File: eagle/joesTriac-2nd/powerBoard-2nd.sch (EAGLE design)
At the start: 43 parts, among them IC1 7809, IC2 7805, IC3 7909, IC5 7809, IC7 LM311N, J1 XF2E-0815-1, J2 XF2E-0815-1

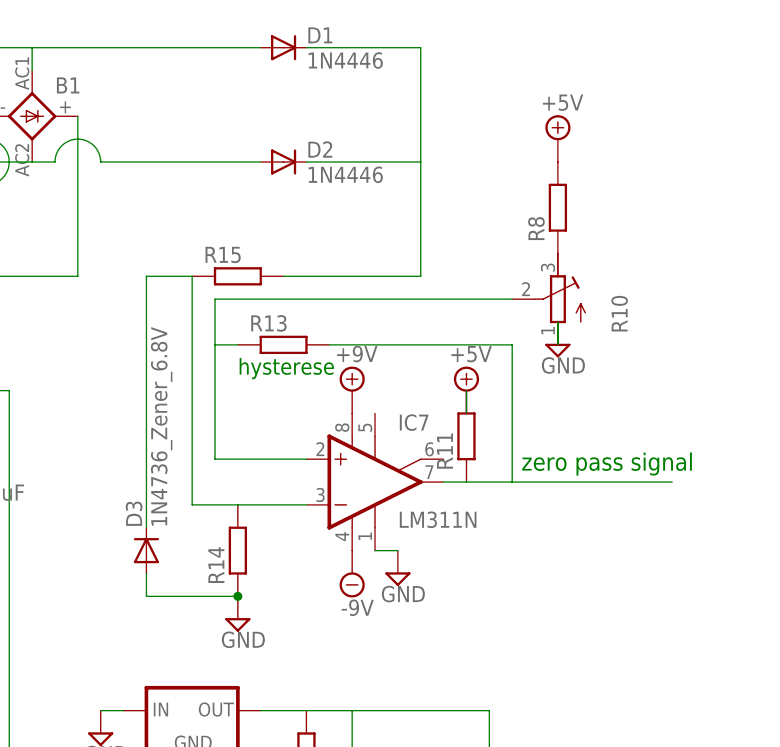
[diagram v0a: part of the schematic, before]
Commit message: reg save
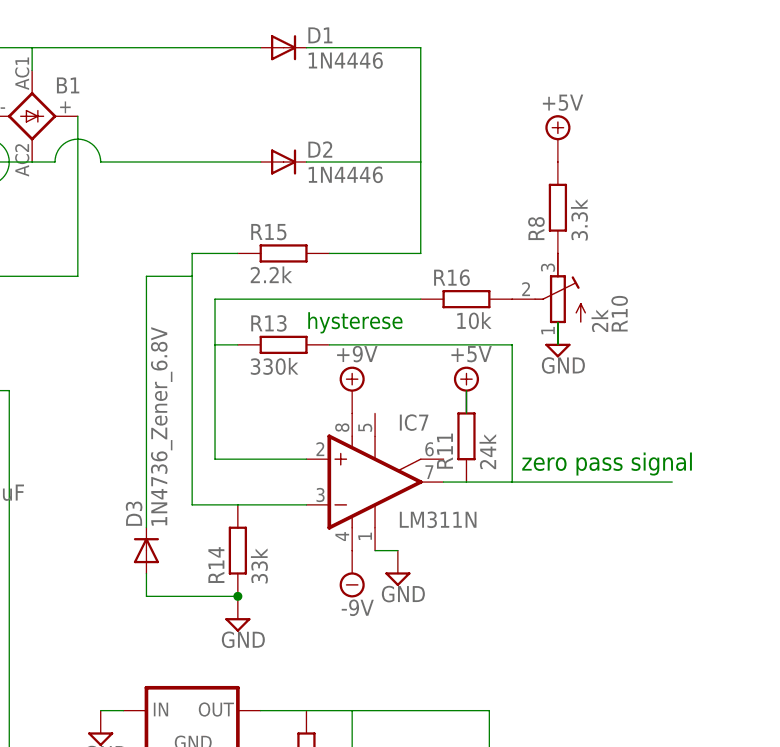
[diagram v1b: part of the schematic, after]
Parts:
- added R16: 10k, resistor:R-EU_0309/V
- R10: value (none) -> 2k
- R11: value (none) -> 24k
- R13: value (none) -> 330k
- R14: value (none) -> 33k
- R15: value (none) -> 2.2k
- R8: value (none) -> 3.3k
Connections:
- new net N$27: R10.S, R16.2
- net N$25: now also R16.1; no longer R10.S
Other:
- moved on the sheet: R15
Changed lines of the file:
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@@
 <part name="D2" library="diode" deviceset="1N4446" device=""/>
 <part name="IC7" library="linear" deviceset="LM311" device="N"/>
-<part name="R8" library="resistor" deviceset="R-EU_" device="0309/V"/>
-<part name="R10" library="resistor" deviceset="R-TRIMM" device="4G/J"/>
+<part name="R8" library="resistor" deviceset="R-EU_" device="0309/V" value="3.3k"/>
+<part name="R10" library="resistor" deviceset="R-TRIMM" device="4G/J" value="2k"/>
 <part name="SUPPLY5" library="supply2" deviceset="+5V" device=""/>
 <part name="SUPPLY17" library="supply2" deviceset="GND" device=""/>
@@
 <part name="SUPPLY19" library="supply2" deviceset="-9V" device=""/>
 <part name="SUPPLY20" library="supply2" deviceset="+5V" device=""/>
-<part name="R11" library="resistor" deviceset="R-EU_" device="0309/V"/>
+<part name="R11" library="resistor" deviceset="R-EU_" device="0309/V" value="24k"/>
 <part name="SUPPLY21" library="supply2" deviceset="GND" device=""/>
-<part name="R13" library="resistor" deviceset="R-EU_" device="0309/V"/>
-<part name="R14" library="resistor" deviceset="R-EU_" device="0309/V"/>
+<part name="R13" library="resistor" deviceset="R-EU_" device="0309/V" value="330k"/>
+<part name="R14" library="resistor" deviceset="R-EU_" device="0309/V" value="33k"/>
 <part name="SUPPLY23" library="supply2" deviceset="GND" device=""/>
-<part name="R15" library="resistor" deviceset="R-EU_" device="0309/V"/>
+<part name="R15" library="resistor" deviceset="R-EU_" device="0309/V" value="2.2k"/>
 <part name="D3" library="diode" deviceset="1N4446" device="" value="1N4736_Zener_6.8V"/>
+<part name="R16" library="resistor" deviceset="R-EU_" device="0309/V" value="10k"/>
 </parts>
 <sheets>
@@
 <text x="-124.46" y="-10.16" size="1.778" layer="91">/-16V</text>
 <text x="46.736" y="46.99" size="1.9304" layer="91">zero pass signal</text>
-<text x="15.24" y="57.658" size="1.778" layer="91">hysterese</text>
+<text x="22.86" y="62.738" size="1.778" layer="91">hysterese</text>
 </plain>
 <instances>
@@
 <instance part="R14" gate="G$1" x="15.24" y="38.1" rot="R90"/>
 <instance part="SUPPLY23" gate="GND" x="15.24" y="30.48"/>
-<instance part="R15" gate="G$1" x="15.24" y="68.58"/>
+<instance part="R15" gate="G$1" x="20.32" y="71.12"/>
 <instance part="D3" gate="1" x="5.08" y="38.1" rot="R90"/>
+<instance part="R16" gate="G$1" x="40.64" y="66.04" smashed="yes">
+<attribute name="NAME" x="36.83" y="67.5386" size="1.778" layer="95"/>
+<attribute name="VALUE" x="39.37" y="62.738" size="1.778" layer="96"/>
+</instance>
 </instances>
 <busses>
@@
 <net name="N$22" class="0">
 <segment>
-<wire x1="10.16" y1="68.58" x2="10.16" y2="43.18" width="0.1524" layer="91"/>
-<wire x1="10.16" y1="43.18" x2="15.24" y2="43.18" width="0.1524" layer="91"/>
+<wire x1="10.16" y1="68.58" x2="5.08" y2="68.58" width="0.1524" layer="91"/>
+<wire x1="5.08" y1="68.58" x2="5.08" y2="40.64" width="0.1524" layer="91"/>
+<pinref part="D3" gate="1" pin="C"/>
 <pinref part="IC7" gate="A" pin="-IN"/>
 <wire x1="15.24" y1="43.18" x2="22.86" y2="43.18" width="0.1524" layer="91"/>
 <pinref part="R14" gate="G$1" pin="2"/>
+<wire x1="10.16" y1="43.18" x2="15.24" y2="43.18" width="0.1524" layer="91"/>
+<wire x1="10.16" y1="68.58" x2="10.16" y2="43.18" width="0.1524" layer="91"/>
 <pinref part="R15" gate="G$1" pin="1"/>
-<wire x1="10.16" y1="68.58" x2="5.08" y2="68.58" width="0.1524" layer="91"/>
-<wire x1="5.08" y1="68.58" x2="5.08" y2="40.64" width="0.1524" layer="91"/>
-<pinref part="D3" gate="1" pin="C"/>
+<wire x1="15.24" y1="71.12" x2="10.16" y2="71.12" width="0.1524" layer="91"/>
+<wire x1="10.16" y1="71.12" x2="10.16" y2="68.58" width="0.1524" layer="91"/>
 </segment>
 </net>
@@
 <net name="N$25" class="0">
 <segment>
-<pinref part="R10" gate="G$1" pin="S"/>
-<wire x1="45.72" y1="66.04" x2="12.7" y2="66.04" width="0.1524" layer="91"/>
+<wire x1="35.56" y1="66.04" x2="12.7" y2="66.04" width="0.1524" layer="91"/>
 <wire x1="12.7" y1="66.04" x2="12.7" y2="60.96" width="0.1524" layer="91"/>
 <wire x1="12.7" y1="60.96" x2="12.7" y2="48.26" width="0.1524" layer="91"/>
-<wire x1="12.7" y1="48.26" x2="22.86" y2="48.26" width="0.1524" layer="91"/>
-<pinref part="IC7" gate="A" pin="+IN"/>
 <pinref part="R13" gate="G$1" pin="1"/>
 <wire x1="15.24" y1="60.96" x2="12.7" y2="60.96" width="0.1524" layer="91"/>
+<pinref part="R16" gate="G$1" pin="1"/>
+<pinref part="IC7" gate="A" pin="+IN"/>
+<wire x1="12.7" y1="48.26" x2="22.86" y2="48.26" width="0.1524" layer="91"/>
 </segment>
 </net>
@@
 <wire x1="22.86" y1="93.98" x2="35.56" y2="93.98" width="0.1524" layer="91"/>
 <wire x1="35.56" y1="93.98" x2="35.56" y2="81.28" width="0.1524" layer="91"/>
-<wire x1="35.56" y1="81.28" x2="35.56" y2="68.58" width="0.1524" layer="91"/>
+<wire x1="35.56" y1="81.28" x2="35.56" y2="71.12" width="0.1524" layer="91"/>
 <wire x1="22.86" y1="81.28" x2="35.56" y2="81.28" width="0.1524" layer="91"/>
 <pinref part="D2" gate="1" pin="C"/>
 <pinref part="R15" gate="G$1" pin="2"/>
-<wire x1="20.32" y1="68.58" x2="35.56" y2="68.58" width="0.1524" layer="91"/>
+<wire x1="25.4" y1="71.12" x2="35.56" y2="71.12" width="0.1524" layer="91"/>
 </segment>
 </net>
@@
 </segment>
 </net>
+<net name="N$27" class="0">
+<segment>
+<pinref part="R10" gate="G$1" pin="S"/>
+<pinref part="R16" gate="G$1" pin="2"/>
+</segment>
+</net>
